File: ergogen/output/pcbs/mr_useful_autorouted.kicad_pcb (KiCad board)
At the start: 2 copper layers, 57 x 95 mm, 37 parts

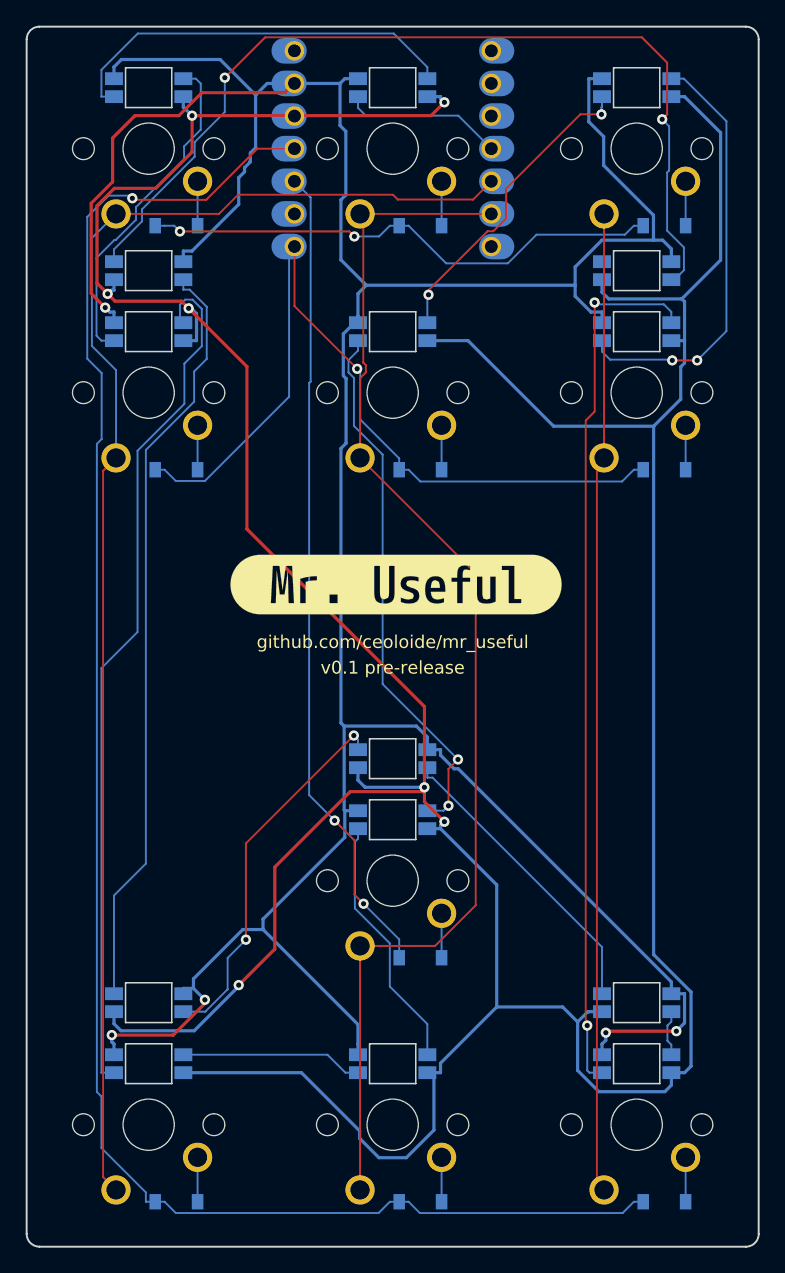
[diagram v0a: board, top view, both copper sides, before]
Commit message: Update assets
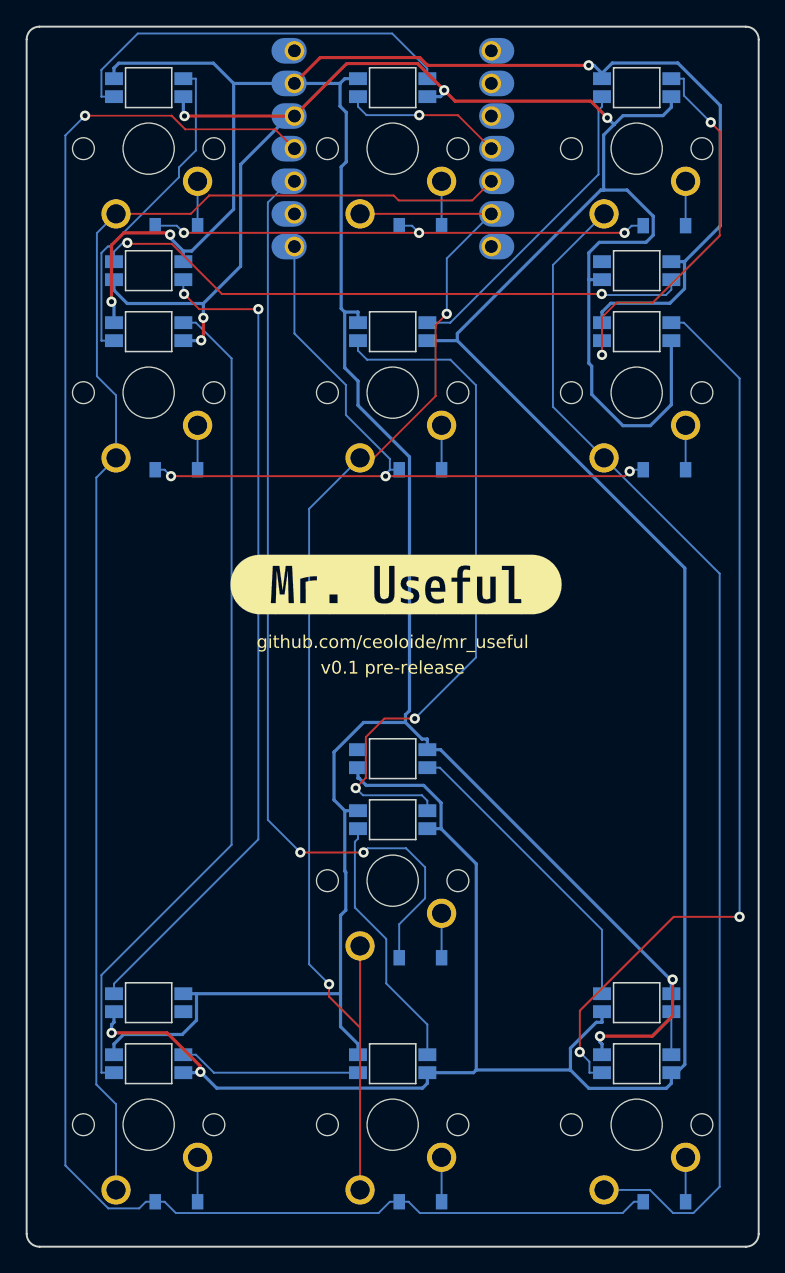
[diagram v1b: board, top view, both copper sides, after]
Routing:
- net VCC: track 333.7 -> 291.1 mm
- net ULED_2: track 29.2 -> 0.00 mm, vias 2 -> 0
- net ULED_4: track 72.9 -> 47.1 mm
- net C2: track 76.5 -> 93.4 mm
- net LED_6: track 42.2 -> 54.5 mm
- net R0: track 138.1 -> 148.2 mm
- net R1: track 64.4 -> 72.7 mm
- net GND: track 269.1 -> 260.8 mm
- net ULED_3: track 59.6 -> 65.4 mm, vias 0 -> 2
- net R3: track 66.1 -> 60.7 mm, vias 1 -> 3
- net LED_8: track 33.8 -> 30.2 mm
- net C1: track 97.8 -> 101.1 mm, vias 0 -> 2
- net LED_9: track 68.5 -> 70.6 mm
- net LED_3: track 67.4 -> 65.7 mm
- net R4: track 41.1 -> 40.2 mm, vias 2 -> 3
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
